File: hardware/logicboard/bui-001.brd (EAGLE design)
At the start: 72 x 72 mm, 28 parts, among them IC1 5V, IC2 74LS07N, IC3 4066N, K1 G5V1, T1 2SC1815, U1 DS18B20

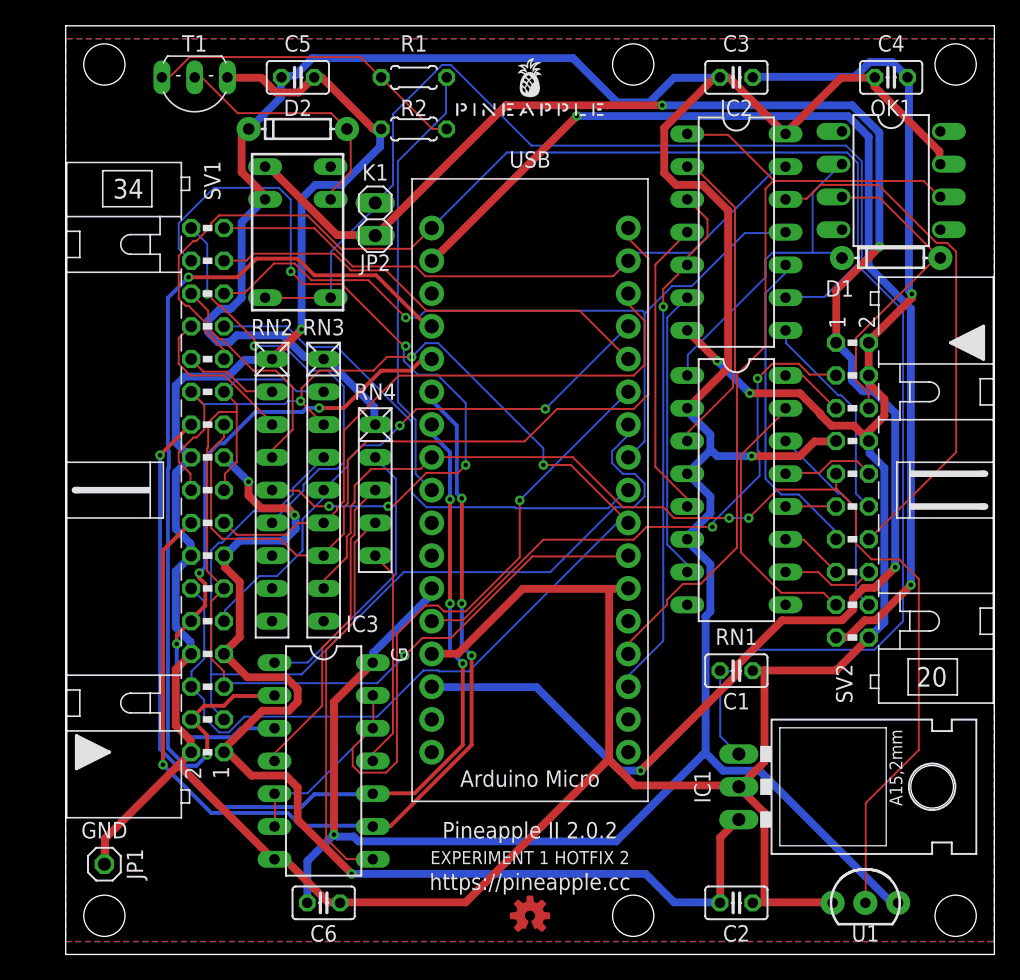
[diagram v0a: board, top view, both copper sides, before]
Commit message: Finished schematic.
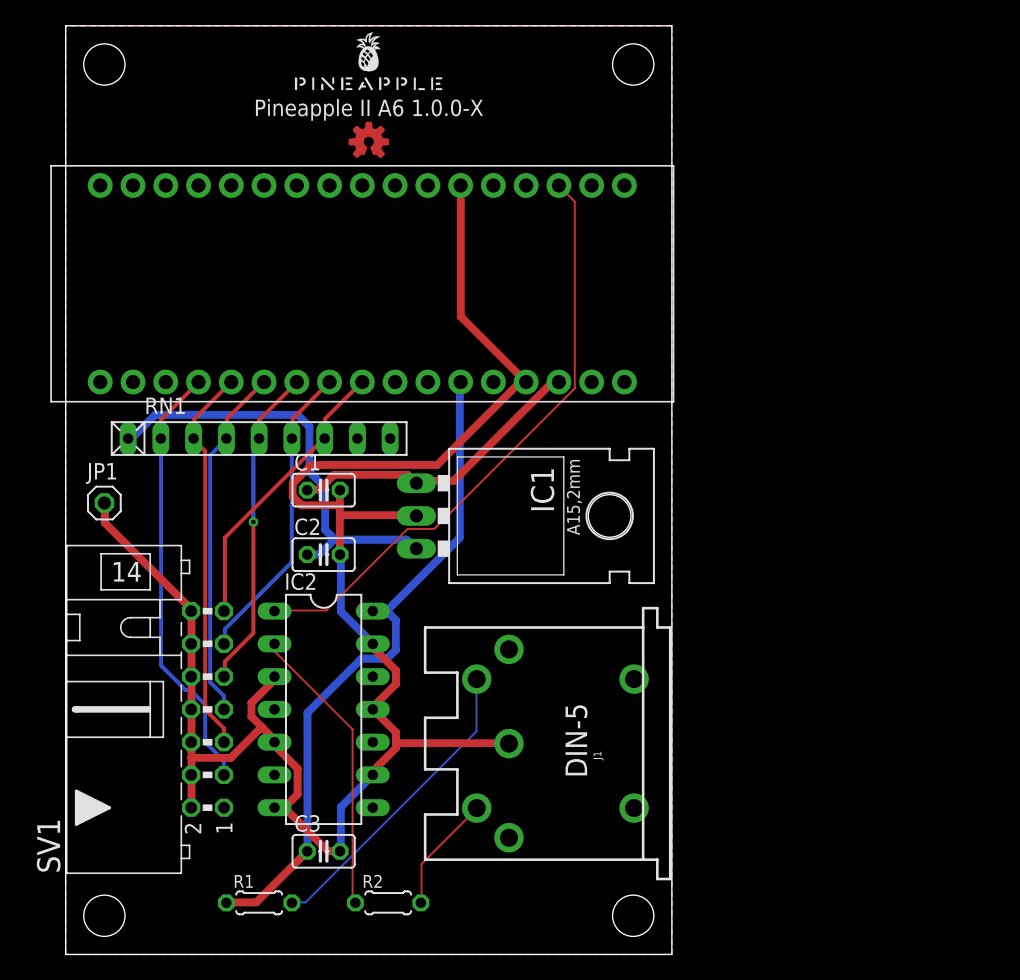
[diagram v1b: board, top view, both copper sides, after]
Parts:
- removed C4, C5, C6: 103, rcl:C025-025X050
- removed D1, D2: (no value), SparkFun-DiscreteSemi:DIODE-1N4148
- removed IC3: 4066N, 40xx:DIL14
- removed JP2: (no value), pinhead:1X02
- removed K1: G5V1, relay:G5V1
- removed OK1: 6N137, optocoupler:DIL08
- removed RN2: 330, resistor-net:RN-9
- removed RN3: 4.7k, resistor-net:RN-9
- removed RN4: 10k, resistor-net:RN-5
- removed SV2: (no value), con-ml:ML20L
- removed T1: 2SC1815, transistor:TO92-ECB
- removed U1: DS18B20, SparkFun-Sensors:TO-92-AMMO
- added J1: DIN5, SparkFun-Connectors:DIN5-RA-PTH
- R1: value 1k -> 220
- R2: value 47k -> 220
- RN1: value 220 -> 10k; device resistor-dil:DIL16 -> resistor-net:RN-9
- SV1: device con-ml:ML34L -> con-ml:ML14L
- moved C3 68.0 mm to (20.0, 8.00)
- moved R1 65.1 mm to (15.0, 4.00)
- moved LOGO1 61.3 mm to (23.5, 63.0)
- moved R2 60.0 mm to (25.0, 4.00)
- moved IC2 48.9 mm to (20.0, 19.0)
- moved C2 41.9 mm to (20.0, 31.0)
- moved RN1 37.2 mm to (15.0, 40.0), turned to 0 degrees
- moved C1 34.9 mm to (20.0, 36.0)
- moved IC1 32.6 mm to (31.0, 34.0)
- moved JP1 28.0 mm to (3.00, 35.0)
- moved MC1 20.6 mm to (23.0, 52.0), turned to 0 degrees
- moved SV1 17.0 mm to (11.0, 19.0)
- moved U$1 12.7 mm to (23.5, 67.0)
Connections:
- removed net 12VRLY: C1.1, IC1.IN, JP2.2, K1.5, K1.6
- removed net A1: IC3.2, MC1.P$31, SV1.4
- removed net A2: IC3.3, MC1.P$30, SV1.10
- removed net A3: IC3.9, MC1.P$29, SV1.16
- removed net A4: IC3.10, MC1.P$28, SV1.22
- removed net D1: MC1.P$7, RN3.4, SV1.3
- removed net D2: MC1.P$4, RN3.5, SV1.9
- removed net D3: MC1.P$3, RN3.6, SV1.15
- removed net D4: MC1.P$1, RN3.7, SV1.21
- removed net LED0: IC2.9, MC1.P$34, SV1.25
- removed net LED0K: RN2.2, SV1.26
- removed net LED1: MC1.P$9, SV1.27
- removed net LED1K: RN2.3, SV1.28
- removed net LED2: IC2.11, MC1.P$8, SV1.29
- removed net LED2K: RN2.4, SV1.30
- removed net LED3: MC1.P$5, SV1.31
- removed net LED3K: RN2.5, SV1.32
- removed net LED4: IC2.13, MC1.P$2, SV1.33
- removed net LED4K: RN2.6, SV1.34
- removed net MIDIINSND: D1.C, OK1.2, RN1.1
- removed net MIDIOUT2RTN: IC2.6, RN1.7
- removed net MIDIOUTRTN: IC2.4, RN1.5
- removed net MIDITHRURTN: IC2.2, RN1.3
- removed net MINRTN: D1.A, OK1.3, SV2.6
- removed net MINSND: RN1.16, SV2.5
- removed net MO1RTN: RN1.12, SV2.11
- removed net MO1SND: RN1.13, SV2.10
- removed net MO2RTN: RN1.10, SV2.16
- removed net MO2SND: RN1.11, SV2.15
- removed net MTHRTN: RN1.14, SV2.18
- removed net MTHSND: RN1.15, SV2.17
- removed net N$3: IC3.1, RN4.2
- removed net N$4: IC3.4, RN4.3
- removed net N$5: IC3.8, RN4.4
- removed net N$6: IC3.11, RN4.5
- removed net PULLUP: IC3.12, IC3.13, IC3.5, IC3.6, MC1.P$6
- removed net RLY: MC1.P$26, R1.2
- removed net RLYDRV: R1.1, R2.2, T1.B
- removed net RLYSNK: D2.A, K1.9, T1.C
- removed net RST: MC1.P$13, SV2.3
- removed net RX: IC2.1, MC1.P$14, OK1.6
- removed net SCL: MC1.P$10, RN3.3, SV1.12, SV1.18, SV1.24, SV1.6
- removed net SDA: MC1.P$11, RN3.2, SV1.11, SV1.17, SV1.23, SV1.5
- removed net THS: MC1.P$27, RN3.8, SV2.9, U1.2
- removed net TX: IC2.3, IC2.5, MC1.P$15
- removed net VDD: MC1.P$33, SV2.19
- removed net XLEDB: IC2.10, SV2.13
- removed net XLEDG: IC2.8, SV2.12
- removed net XLEDR: IC2.12, SV2.14
- new net ANALOG0: MC1.P$31, RN1.2, SV1.3
- new net ANALOG1: MC1.P$30, RN1.3, SV1.5
- new net ANALOG2: MC1.P$29, RN1.4, SV1.7
- new net ANALOG3: MC1.P$28, RN1.5, SV1.9
- new net ANALOG4: MC1.P$27, RN1.6, SV1.11
- new net ANALOG5: MC1.P$26, RN1.7, SV1.13
- new net N$10: J1.4, R1.2
- new net N$7: IC2.1, MC1.P$15
- new net N$8: IC2.2, R2.1
- new net N$9: J1.5, R2.2
- net +12V: now also C1.1, IC1.IN; no longer JP2.1, K1.1, SV2.1
- net GND: now also IC2.11, IC2.13, IC2.3, IC2.5, IC2.9, J1.2, SV1.10, SV1.12, SV1.4, SV1.6; no longer C4.2, C5.2, C6.2, IC3.7, R2.1, RN2.1, SV1.20, SV2.2, SV2.20, SV2.4, SV2.8, T1.E, U1.1
- net VCC: now also R1.1; no longer C4.1, C5.1, C6.1, D2.C, IC3.14, K1.2, OK1.7, RN1.2, RN1.4, RN1.6, RN3.1, RN4.1, SV2.7, U1.3
- net VOUT: now also RN1.1; no longer SV1.1, SV1.13, SV1.19, SV1.7
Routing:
- net VCC: track 255.8 -> 53.1 mm, vias 2 -> 0
- net GND: track 286.3 -> 144.4 mm, vias 4 -> 0
- net 12VRLY: track 122.2 -> 0.00 mm
- net +12V: track 138.4 -> 23.5 mm, vias 4 -> 0
- net SCL: track 106.7 -> 0.00 mm, vias 3 -> 0
- net THS: track 89.0 -> 0.00 mm, vias 2 -> 0
- net VDD: track 82.8 -> 0.00 mm, vias 2 -> 0
- net LED0: track 82.7 -> 0.00 mm
- net A4: track 79.4 -> 0.00 mm, vias 4 -> 0
- net SDA: track 77.0 -> 0.00 mm, vias 1 -> 0
- net A3: track 76.9 -> 0.00 mm, vias 4 -> 0
- net A1: track 73.4 -> 0.00 mm, vias 2 -> 0
- net D1: track 72.5 -> 0.00 mm
- net D4: track 65.2 -> 0.00 mm
- net RX: track 63.8 -> 0.00 mm
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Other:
- board size 72 x 72 mm -> 47 x 72 mm
- board text added: "Pineapple II A6 1.0.0-X"
- board text removed: "Arduino Micro"
- board text removed: "EXPERIMENT 1 HOTFIX 2"
- board text removed: "G"
- board text removed: "GND"
- board text removed: "Pineapple II 2.0.2"
- board text removed: "USB"
- board text removed: "https://pineapple.cc"
